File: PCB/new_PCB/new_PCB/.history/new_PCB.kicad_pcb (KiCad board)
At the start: 2 copper layers, 134.6 x 68.6 mm, 32 parts, among them J1 XT60PW-F, J2 XT60PW-F, J3 MOLEX-Connector, J4 MOLEX-Connector, J5 MOLEX-Connector, J6 MOLEX-Connector, J7 MOLEX-Connector, J8 MOLEX-Connector, Q1 Q_PMOS, Q2 Q_PMOS, U1 ESP32-S3-DEVKITC-1-N16R8V

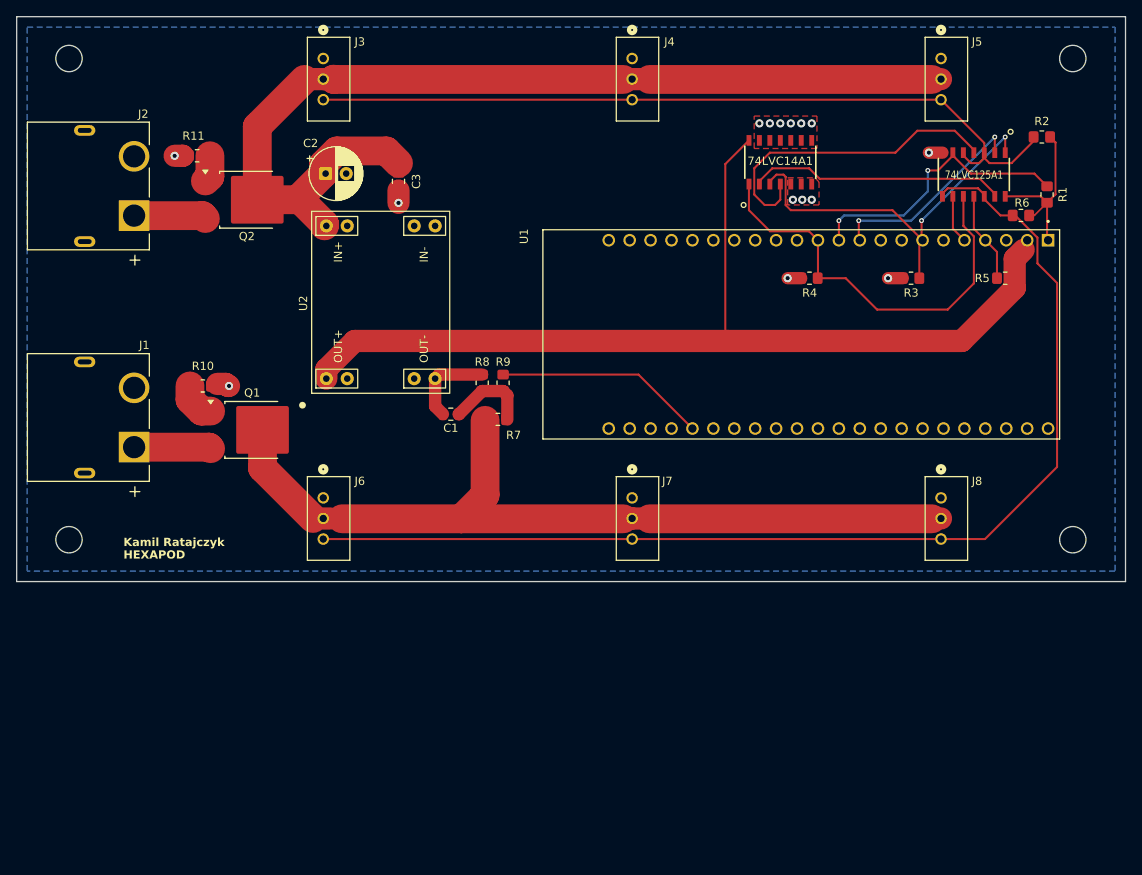
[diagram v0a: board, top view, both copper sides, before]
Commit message: Final version of 2.0 PCB version
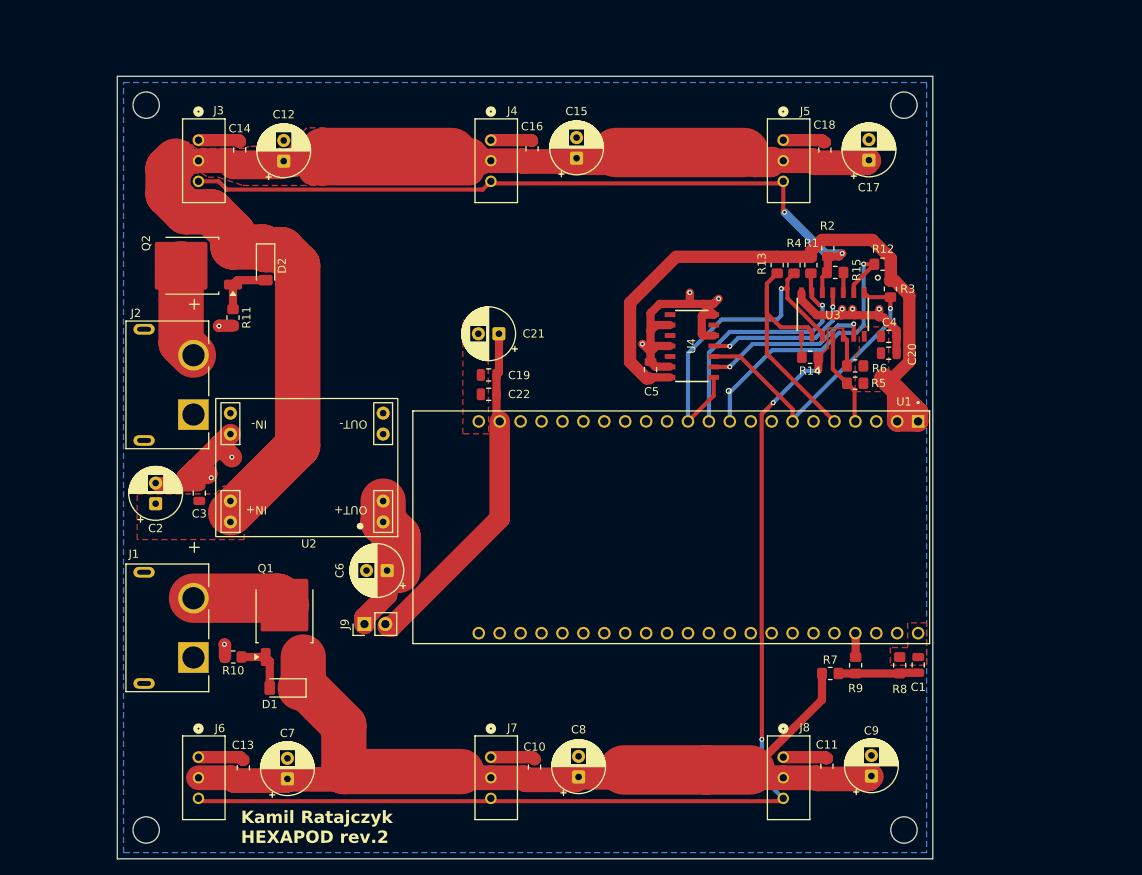
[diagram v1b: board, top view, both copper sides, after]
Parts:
- removed 74LVC125A1, 74LVC14A1: ~, Elements:SOT108-1
- added C10: 100nF, Capacitor_SMD:C_0805_2012Metric, F.Cu at (80.6, 107.6)
- added C11: 100nF, Capacitor_SMD:C_0805_2012Metric, F.Cu at (116.2, 107.5)
- added C12: 220uF, Capacitor_THT:CP_Radial_D6.3mm_P2.50mm, F.Cu at (50.2, 34.0)
- added C13: 100nF, Capacitor_SMD:C_0805_2012Metric, F.Cu at (45.3, 107.7)
- added C14: 100nF, Capacitor_SMD:C_0805_2012Metric, F.Cu at (44.9, 32.7)
- added C15: 220uF, Capacitor_THT:CP_Radial_D6.3mm_P2.50mm, F.Cu at (85.8, 33.7)
- added C16: 100nF, Capacitor_SMD:C_0805_2012Metric, F.Cu at (80.4, 32.5)
- added C17: 220uF, Capacitor_THT:CP_Radial_D6.3mm_P2.50mm, F.Cu at (121.2, 33.9)
- added C18: 100nF, Capacitor_SMD:C_0805_2012Metric, F.Cu at (115.9, 32.7)
- added C19: 10uF, Capacitor_SMD:C_0805_2012Metric, F.Cu at (75.1, 60.0)
- added C20: 10uF, Capacitor_SMD:C_0805_2012Metric, F.Cu at (123.7, 57.4)
- added C21: 220uF, Capacitor_THT:CP_Radial_D6.3mm_P2.50mm, F.Cu at (76.3, 55.0)
- added C22: 100nF, Capacitor_SMD:C_0805_2012Metric, F.Cu at (75.1, 62.4)
- added C4: 100nF, Capacitor_SMD:C_0805_2012Metric, F.Cu at (123.7, 55.3)
- added C5: 100nF, Capacitor_SMD:C_0805_2012Metric, F.Cu at (94.7, 59.4)
- added C6: 22uF, Capacitor_THT:CP_Radial_D6.3mm_P2.50mm, F.Cu at (62.8, 83.8)
- added C7: 220uF, Capacitor_THT:CP_Radial_D6.3mm_P2.50mm, F.Cu at (50.6, 109.0)
- added C8: 220uF, Capacitor_THT:CP_Radial_D6.3mm_P2.50mm, F.Cu at (86.0, 108.8)
- added C9: 220uF, Capacitor_THT:CP_Radial_D6.3mm_P2.50mm, F.Cu at (121.5, 108.7)
- added D1: BZV55B15, Diode_SMD:D_MiniMELF, F.Cu at (50.2, 98.0)
- added D2: BZV55B15, Diode_SMD:D_MiniMELF, F.Cu at (48.0, 46.8)
- added J9: Conn_01x02, Connector_PinHeader_2.54mm:PinHeader_1x02_P2.54mm_Vertical, F.Cu at (60.0, 90.2)
- added R12: 10k, Resistor_SMD:R_0805_2012Metric_Pad1.20x1.40mm_HandSolder, F.Cu at (122.9, 46.6)
- added R13: 10k, Resistor_SMD:R_0805_2012Metric_Pad1.20x1.40mm_HandSolder, F.Cu at (110.1, 46.7)
- added R14: 22R, Resistor_SMD:R_0805_2012Metric_Pad1.20x1.40mm_HandSolder, F.Cu at (114.1, 57.9)
- added R15: 22R, Resistor_SMD:R_0805_2012Metric_Pad1.20x1.40mm_HandSolder, F.Cu at (117.2, 47.6)
- added U3: 74LVC125A1, Elements:SOT108-1, F.Cu at (120.7, 50.0)
- added U4: 74LVC14A1, Elements:SOT108-1, F.Cu at (102.4, 60.3)
- Q1, Q2: value Q_PMOS -> SUD50P04-08
- moved H1 146.4 mm to (33.5, 115.2)
- moved H2 138.0 mm to (125.5, 115.2)
- moved C1 64.4 mm to (127.2, 95.2), turned to 90 degrees
- moved R8 61.2 mm to (125.0, 95.3)
- moved H3 56.6 mm to (125.5, 27.2)
- moved R9 54.8 mm to (119.6, 95.3)
- moved H4 53.6 mm to (33.5, 27.2)
- moved R7 50.8 mm to (116.5, 96.2)
- moved C2 45.1 mm to (34.6, 75.6), turned to 90 degrees
- moved C3 44.9 mm to (40.0, 74.3), turned to 90 degrees
- moved J8 36.8 mm to (110.8, 106.4)
- moved J7 35.8 mm to (75.3, 106.4)
- moved J6 34.9 mm to (39.8, 106.4)
- moved R10 33.1 mm to (44.1, 94.2), turned to 180 degrees
- moved R1 29.9 mm to (114.2, 46.7), turned to -90 degrees
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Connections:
- net Net-(C1-Pad1) renamed /BAT_LVL_DIV
- net Net-(Q1-G) renamed /Q1_GATE
- net Net-(Q2-G) renamed /Q2_GATE
- J1 pad 1: VBAT -> VBAT_1
- J2 pad 1: VBAT -> VBAT_2
- Q1 pad 2: VBUS_1 -> VBAT_1
- Q1 pad 3: VBAT -> VBUS_1
- Q2 pad 2: VBUS_2 -> VBAT_2
- Q2 pad 3: VBAT -> VBUS_2
- R1 pad 1: +3.3V -> +3V3
- R2 pad 1: +3.3V -> +3V3
- R3 pad 1: /TXEN1 -> +3V3
- R3 pad 2: GND -> /TXEN1
- R4 pad 1: /TXEN2 -> +3V3
- R4 pad 2: GND -> /TXEN2
- R5 pad 1: +3.3V -> +3V3
- R6 pad 1: +3.3V -> +3V3
- U1 pad J1_1: +3.3V -> +3V3
- U1 pad J1_2: +3.3V -> +3V3
- U1 pad J1_21: unconnected-(U1-5V0-PadJ1_21) -> +5V
- U1 pad J3_18: /BAT_LVL -> unconnected-(U1-GPIO21-PadJ3_18)
- U1 pad J3_4: unconnected-(U1-GPIO1-PadJ3_4) -> /BAT_LVL
- U2 pad 1: +3.3V -> /+5V_RAW
- U2 pad 2: unconnected-(U2-OUT+-Pad2) -> /+5V_RAW
- U2 pad 3: unconnected-(U2-OUT--Pad3) -> GND
- U2 pad 6: unconnected-(U2-IN--Pad6) -> GND
- U2 pad 7: unconnected-(U2-IN+-Pad7) -> VBUS_2
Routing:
- net +3.3V: track 146.5 -> 0.00 mm
- net GND: track 19.8 -> 109.6 mm, vias 15 -> 10
- net +3V3: track 0.00 -> 80.3 mm
- net +5V: track 0.00 -> 41.7 mm
- net VBUS_2: track 119.6 -> 158.9 mm
- net /TX2: track 5.91 -> 31.9 mm
- net /BAT_LVL: track 25.7 -> 2.91 mm
- net VBUS_1: track 100.1 -> 121.0 mm
- net /RXEN1: track 38.9 -> 19.1 mm, vias 0 -> 2
- net VBAT: track 18.2 -> 0.00 mm
- net /+5V_RAW: track 0.00 -> 16.8 mm
- net VBAT_2: track 0.00 -> 11.7 mm
- net VBAT_1: track 0.00 -> 11.6 mm
- net /TX1: track 25.1 -> 36.4 mm, vias 2 -> 1
- net /TXEN1: track 48.0 -> 37.1 mm, vias 2 -> 1
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- added copper zone on F.Cu, net +3V3
- added copper zone on F.Cu, net VBUS_2
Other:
- board size 134.6 x 68.6 mm -> 99 x 95 mm
- board text added: "Kamil Ratajczyk HEXAPOD rev.2"
- board text removed: "HEXAPOD"
- board text removed: "Kamil Ratajczyk"
